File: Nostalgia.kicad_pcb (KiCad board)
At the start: 2 copper layers, 71 x 102 mm, 58 parts, among them J10 490107670612, J20 USB-C6, K1 CONFIG, K10 CONFIG, K11 CONFIG, K12 CONFIG, K13 TACT_6x6_SMD, K14 TACT_6x6_SMD, K15 TACT_6x6_SMD, K16 TACT_6x6_SMD, K2 CONFIG, K3 CONFIG, K4 CONFIG, K5 CONFIG, K6 CONFIG, K7 CONFIG, K8 CONFIG, K9 CONFIG, U1 TP4056, U2 TPS63000, U40 ESP32-S3-WROOM-1-N16R8, U5 TPS613222ADBV

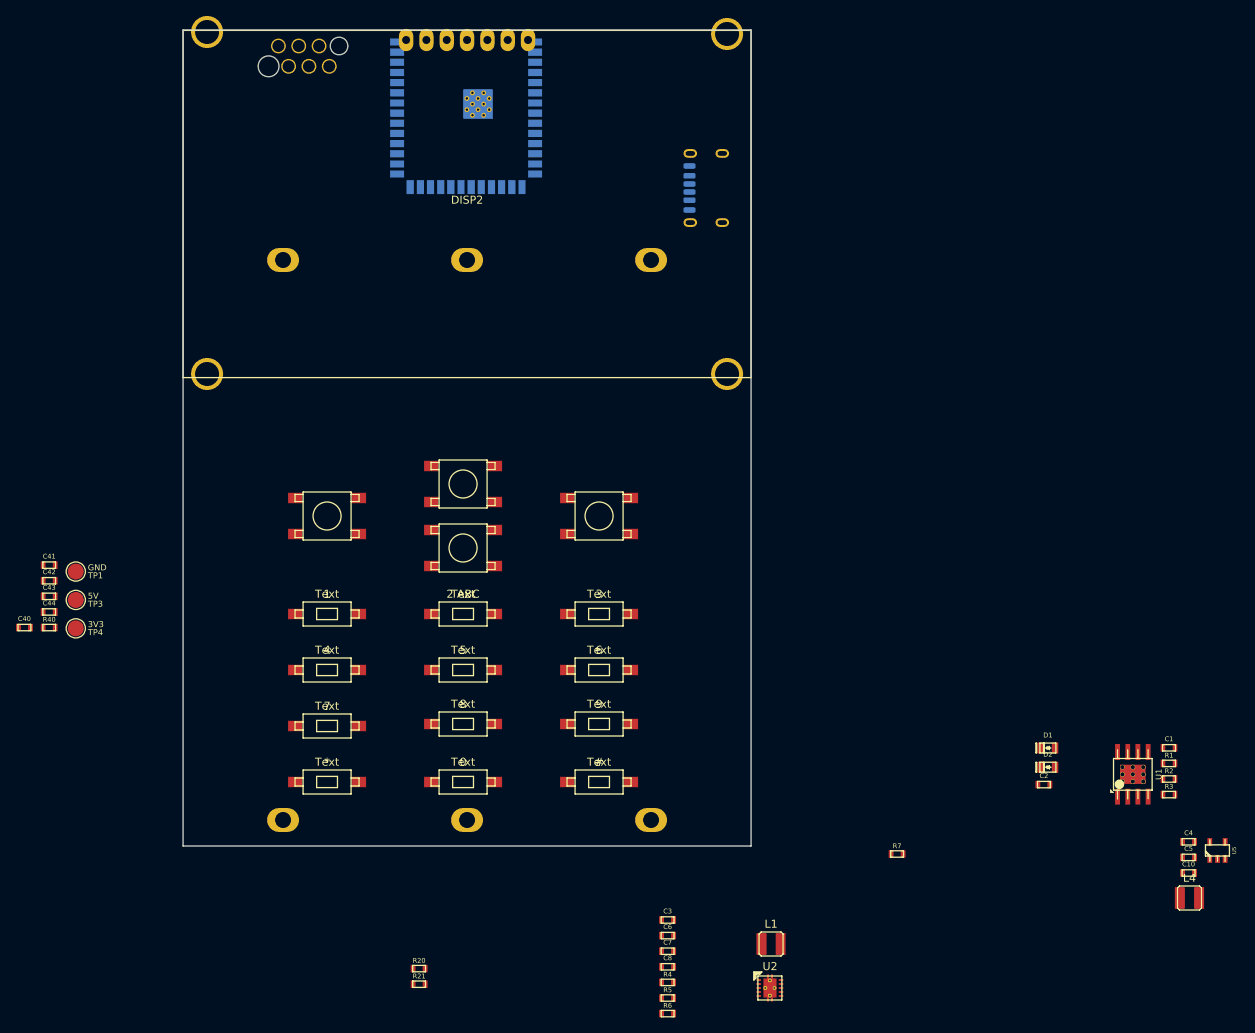
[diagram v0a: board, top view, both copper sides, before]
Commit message: WIP
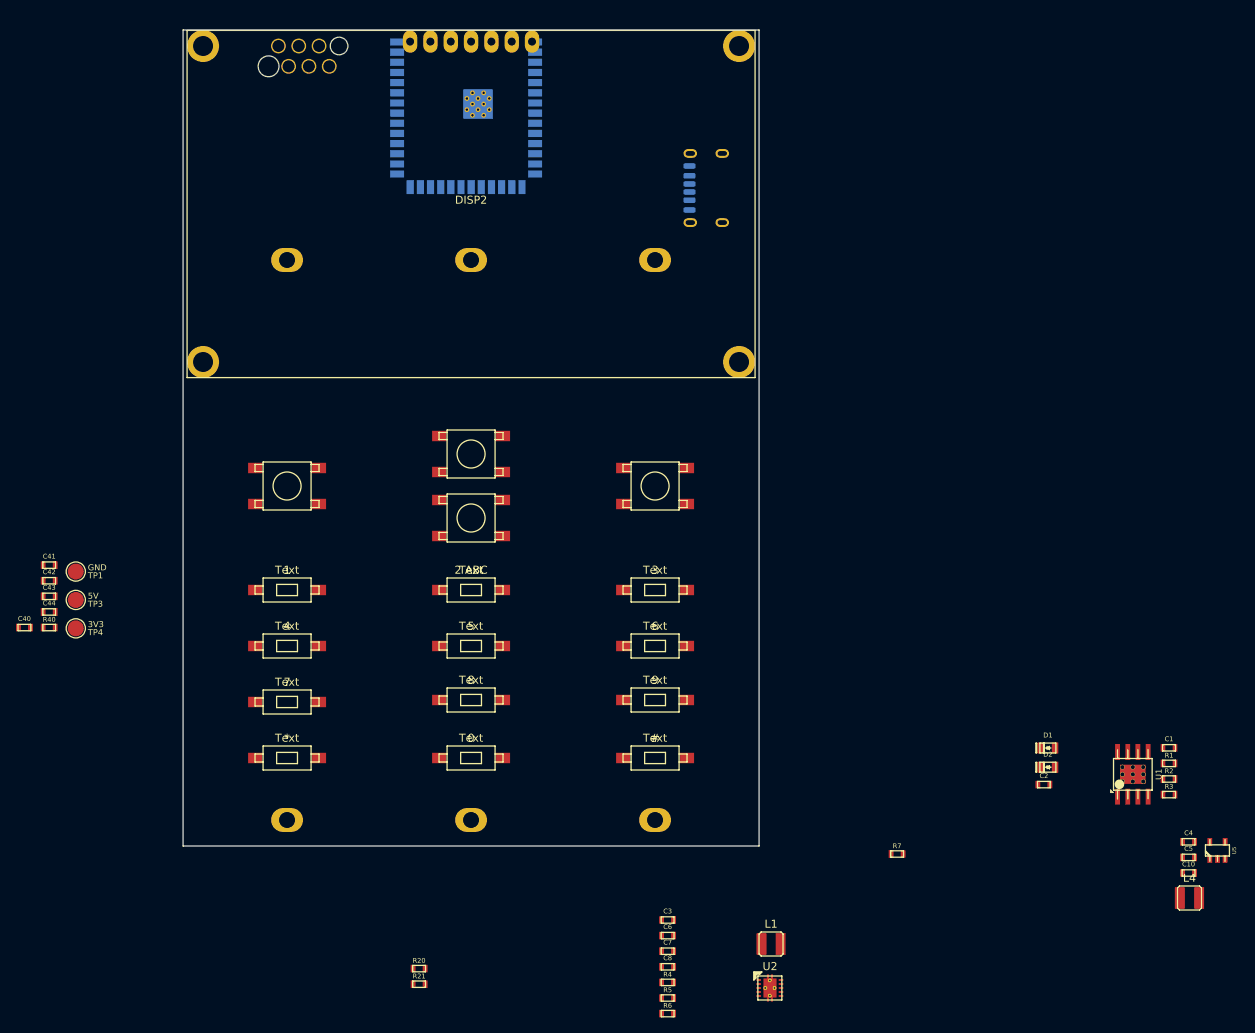
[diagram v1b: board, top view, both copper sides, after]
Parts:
- moved K16 7.94 mm to (59.0, -45.0)
- moved K12 7.62 mm to (59.0, -11.0)
- moved K3 7.62 mm to (59.0, -32.0)
- moved K6 7.62 mm to (59.0, -25.0)
- moved K9 7.62 mm to (59.0, -18.2)
- moved K13 6.25 mm to (13.0, -45.0)
- moved K1 5.83 mm to (13.0, -32.0)
- moved K10 5.83 mm to (13.0, -11.0)
- moved K4 5.83 mm to (13.0, -25.0)
- moved K7 5.83 mm to (13.0, -18.0)
- moved K14 3.88 mm to (36.0, -49.0)
- moved K15 3.88 mm to (36.0, -41.0)
- moved K11 3.16 mm to (36.0, -11.0)
- moved K2 3.16 mm to (36.0, -32.0)
- moved K5 3.16 mm to (36.0, -25.0)
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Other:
- board size 71 x 102 mm -> 72 x 102 mm
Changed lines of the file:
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@@
 	(footprint "_custom:TACT_6x3_SMD"
 		(layer "F.Cu")
-		(at 35 -8)
+		(at 36 -11)
 		(descr "SMD Pushbutton")
 		(property "Reference" "K11"
@@
 	(footprint "_custom:TACT_6x3_SMD"
 		(layer "F.Cu")
-		(at 52 -22)
+		(at 59 -25)
 		(descr "SMD Pushbutton")
 		(property "Reference" "K6"
@@
 	(footprint "_custom:TACT_6x3_SMD"
 		(layer "F.Cu")
-		(at 35 -15.25)
+		(at 36 -18.25)
 		(descr "SMD Pushbutton")
 		(property "Reference" "K8"
@@
 	(footprint "_custom:TACT_6x6_SMD"
 		(layer "F.Cu")
-		(at 35 -45.25 180)
+		(at 36 -49 180)
 		(descr "C&K Components SPST SMD PTS645 Series 6mm Tact Switch")
 		(tags "SPST Button Switch")
@@
 	(footprint "_custom:TACT_6x3_SMD"
 		(layer "F.Cu")
-		(at 18 -8)
+		(at 13 -11)
 		(descr "SMD Pushbutton")
 		(property "Reference" "K10"
@@
 	(footprint "_custom:TACT_6x3_SMD"
 		(layer "F.Cu")
-		(at 35 -22)
+		(at 36 -25)
 		(descr "SMD Pushbutton")
 		(property "Reference" "K5"
@@
 	(footprint "_custom:TACT_6x3_SMD"
 		(layer "F.Cu")
-		(at 18 -15)
+		(at 13 -18)
 		(descr "SMD Pushbutton")
 		(property "Reference" "K7"
@@
 	(footprint "_custom:TACT_6x6_SMD"
 		(layer "F.Cu")
-		(at 52 -41.25)
+		(at 59 -45)
 		(descr "C&K Components SPST SMD PTS645 Series 6mm Tact Switch")
 		(tags "SPST Button Switch")
@@
 	(footprint "_custom:TACT_6x6_SMD"
 		(layer "F.Cu")
-		(at 35 -37.25)
+		(at 36 -41)
 		(descr "C&K Components SPST SMD PTS645 Series 6mm Tact Switch")
 		(tags "SPST Button Switch")
@@
 	(footprint "_custom:TACT_6x3_SMD"
 		(layer "F.Cu")
-		(at 18 -22)
+		(at 13 -25)
 		(descr "SMD Pushbutton")
 		(property "Reference" "K4"
@@
 	(footprint "_custom:OLED_2.42inch_board_2"
 		(layer "F.Cu")
-		(at 35.5 -80.25)
+		(at 36 -80.25)
 		(property "Reference" "DISP2"
 			(at 0 -0.5 0)
@@
 		)
 		(fp_line
-			(start -31 -19.5)
-			(end -31 19.5)
+			(start -31 -18.8)
+			(end -31 20.2)
 			(stroke
 				(width 0.1)
@@
 		)
 		(fp_line
-			(start -19 19.5)
-			(end -31 19.5)
+			(start -19 20.2)
+			(end -31 20.2)
 			(stroke
 				(width 0.1)
@@
 		)
 		(fp_line
-			(start -19 19.5)
-			(end -18 20.5)
+			(start -19 20.2)
+			(end -18 21.2)
 			(stroke
 				(width 0.1)
@@
 		)
 		(fp_line
-			(start -18 20.5)
-			(end 18 20.5)
+			(start -18 21.2)
+			(end 18 21.2)
 			(stroke
 				(width 0.1)
@@
 		)
 		(fp_line
-			(start 19 19.5)
-			(end 18 20.5)
+			(start 19 20.2)
+			(end 18 21.2)
 			(stroke
 				(width 0.1)
@@
 		)
 		(fp_line
-			(start 31 -19.5)
-			(end -31 -19.5)
+			(start 31 -18.8)
+			(end -31 -18.8)
 			(stroke
 				(width 0.1)
@@
 		)
 		(fp_line
-			(start 31 19.5)
-			(end 19 19.5)
+			(start 31 20.2)
+			(end 19 20.2)
 			(stroke
 				(width 0.1)
@@
 		)
 		(fp_line
-			(start 31 19.5)
-			(end 31 -19.5)
+			(start 31 20.2)
+			(end 31 -18.8)
 			(stroke
 				(width 0.1)
@@
 		)
 		(fp_rect
-			(start -28.75 -17.5)
-			(end 28.75 12)
+			(start -28.75 -16.8)
+			(end 28.75 12.7)
 			(stroke
 				(width 0.1)
@@
 		)
 		(pad "1" thru_hole circle
-			(at -32.5 -21.5)
+			(at -33.5 -19.75)
 			(size 4 4)
-			(drill 3)
+			(drill 2.5)
 			(layers "*.Cu" "*.Mask")
 			(remove_unused_layers no)
@@
 		)
 		(pad "1" thru_hole circle
-			(at -32.5 21.25)
+			(at -33.5 19.75)
 			(size 4 4)
-			(drill 3)
+			(drill 2.5)
 			(layers "*.Cu" "*.Mask")
 			(remove_unused_layers no)
@@
 		)
 		(pad "1" thru_hole oval
-			(at 7.62 -20.5 90)
+			(at 7.62 -20.3 90)
 			(size 2.8 1.8)
 			(drill 1)
@@
 		)
 		(pad "1" thru_hole circle
-			(at 32.5 -21.25)
+			(at 33.5 -19.75)
 			(size 4 4)
-			(drill 3)
+			(drill 2.5)
 			(layers "*.Cu" "*.Mask")
 			(remove_unused_layers no)
@@
 		)
 		(pad "1" thru_hole circle
-			(at 32.5 21.25)
+			(at 33.5 19.75)
 			(size 4 4)
-			(drill 3)
+			(drill 2.5)
 			(layers "*.Cu" "*.Mask")
 			(remove_unused_layers no)
@@
 		)
 		(pad "2" thru_hole oval
-			(at 5.08 -20.5 90)
+			(at 5.08 -20.3 90)
 			(size 2.8 1.8)
 			(drill 1)
@@
 		)
 		(pad "3" thru_hole oval
-			(at 2.54 -20.5 90)
+			(at 2.54 -20.3 90)
 			(size 2.8 1.8)
 			(drill 1)
@@
 		)
 		(pad "4" thru_hole oval
-			(at 0 -20.5 90)
+			(at 0 -20.3 90)
 			(size 2.8 1.8)
 			(drill 1)
@@
 		)
 		(pad "5" thru_hole oval
-			(at -2.54 -20.5 90)
+			(at -2.54 -20.3 90)
 			(size 2.8 1.8)
 			(drill 1)
@@
 		)
 		(pad "6" thru_hole oval
-			(at -5.08 -20.5 90)
+			(at -5.08 -20.3 90)
 			(size 2.8 1.8)
 			(drill 1)
@@
 		)
 		(pad "7" thru_hole oval
-			(at -7.62 -20.5 90)
+			(at -7.62 -20.3 90)
 			(size 2.8 1.8)
 			(drill 1)
@@
 	(footprint "_custom:TACT_6x3_SMD"
 		(layer "F.Cu")
-		(at 18 -29)
+		(at 13 -32)
 		(descr "SMD Pushbutton")
 		(property "Reference" "K1"
@@
 	(footprint "_custom:TACT_6x3_SMD"
 		(layer "F.Cu")
-		(at 52 -29)
+		(at 59 -32)
 		(descr "SMD Pushbutton")
 		(property "Reference" "K3"
@@
 	(footprint "_custom:TACT_6x3_SMD"
 		(layer "F.Cu")
-		(at 35 -29)
+		(at 36 -32)
 		(descr "SMD Pushbutton")
 		(property "Reference" "K2"
@@
 	(footprint "_custom:TACT_6x3_SMD"
 		(layer "F.Cu")
-		(at 52 -15.25)
+		(at 59 -18.25)
 		(descr "SMD Pushbutton")
 		(property "Reference" "K9"
@@
 	(footprint "_custom:TACT_6x3_SMD"
 		(layer "F.Cu")
-		(at 52 -8)
+		(at 59 -11)
 		(descr "SMD Pushbutton")
 		(property "Reference" "K12"
@@
 	(footprint "_custom:TACT_6x6_SMD"
 		(layer "F.Cu")
-		(at 18 -41.25)
+		(at 13 -45)
 		(descr "C&K Components SPST SMD PTS645 Series 6mm Tact Switch")
 		(tags "SPST Button Switch")
@@
 	(footprint "_custom:Bat_BH-18650-A1AJ005"
 		(layer "B.Cu")
-		(at 35.5 -38.25 90)
+		(at 36 -38.25 90)
 		(property "Reference" "BAT2"
 			(at 39 0 0)
@@
 	(footprint "_custom:Bat_BH-18650-A1AJ005"
 		(layer "B.Cu")
-		(at 12.5 -38.25 90)
+		(at 13 -38.25 90)
 		(property "Reference" "BAT1"
 			(at 39 0 0)
@@
 	(footprint "_custom:Bat_BH-18650-A1AJ005"
 		(layer "B.Cu")
-		(at 58.5 -38.25 90)
+		(at 59 -38.25 90)
 		(property "Reference" "BAT3"
 			(at 39 0 0)
@@
 	(gr_line
 		(start 0 0)
-		(end 71 0)
+		(end 72 0)
 		(stroke
 			(width 0.1)
@@
 	)
 	(gr_line
-		(start 71 0)
-		(end 71 -102)
+		(start 72 0)
+		(end 72 -102)
 		(stroke
 			(width 0.1)
@@
 	)
 	(gr_line
-		(start 71 -102)
+		(start 72 -102)
 		(end 0 -102)
 		(stroke
